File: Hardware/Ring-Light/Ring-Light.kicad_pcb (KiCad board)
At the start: 2 copper layers, 132 x 132 mm, 154 parts, among them Q1 MMBT3904, Q10 MMBT3904, Q11 MMBT3904, Q12 MMBT3904, Q13 MMBT3904, Q14 MMBT3904, Q15 MMBT3904, Q16 MMBT3904, Q2 MMBT3904, Q3 MMBT3904, Q4 MMBT3904, Q5 MMBT3904, Q6 MMBT3904, Q7 MMBT3904, Q8 MMBT3904, Q9 MMBT3904, U1 TPS92612QDBVRQ1, U10 TPS92612QDBVRQ1, U11 TPS92612QDBVRQ1, U12 TPS92612QDBVRQ1, U13 TPS92612QDBVRQ1, U14 TPS92612QDBVRQ1, U15 TPS92612QDBVRQ1, U16 TPS92612QDBVRQ1, U2 TPS92612QDBVRQ1, U3 TPS92612QDBVRQ1, U4 TPS92612QDBVRQ1, U5 TPS92612QDBVRQ1, U6 TPS92612QDBVRQ1, U7 TPS92612QDBVRQ1, U8 TPS92612QDBVRQ1, U9 TPS92612QDBVRQ1

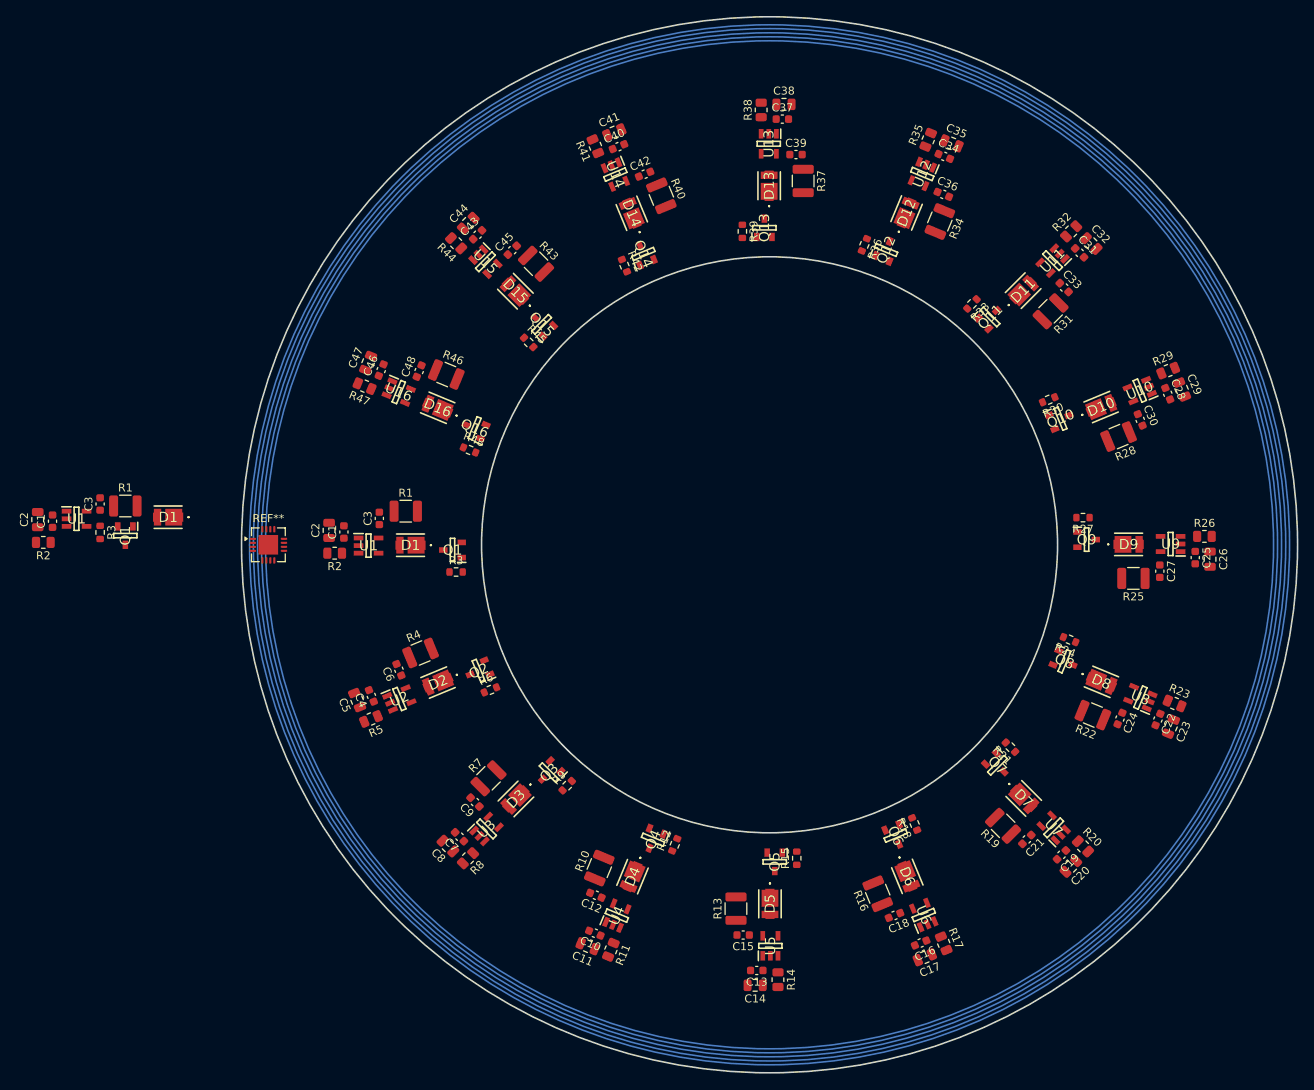
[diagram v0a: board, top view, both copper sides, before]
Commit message: m
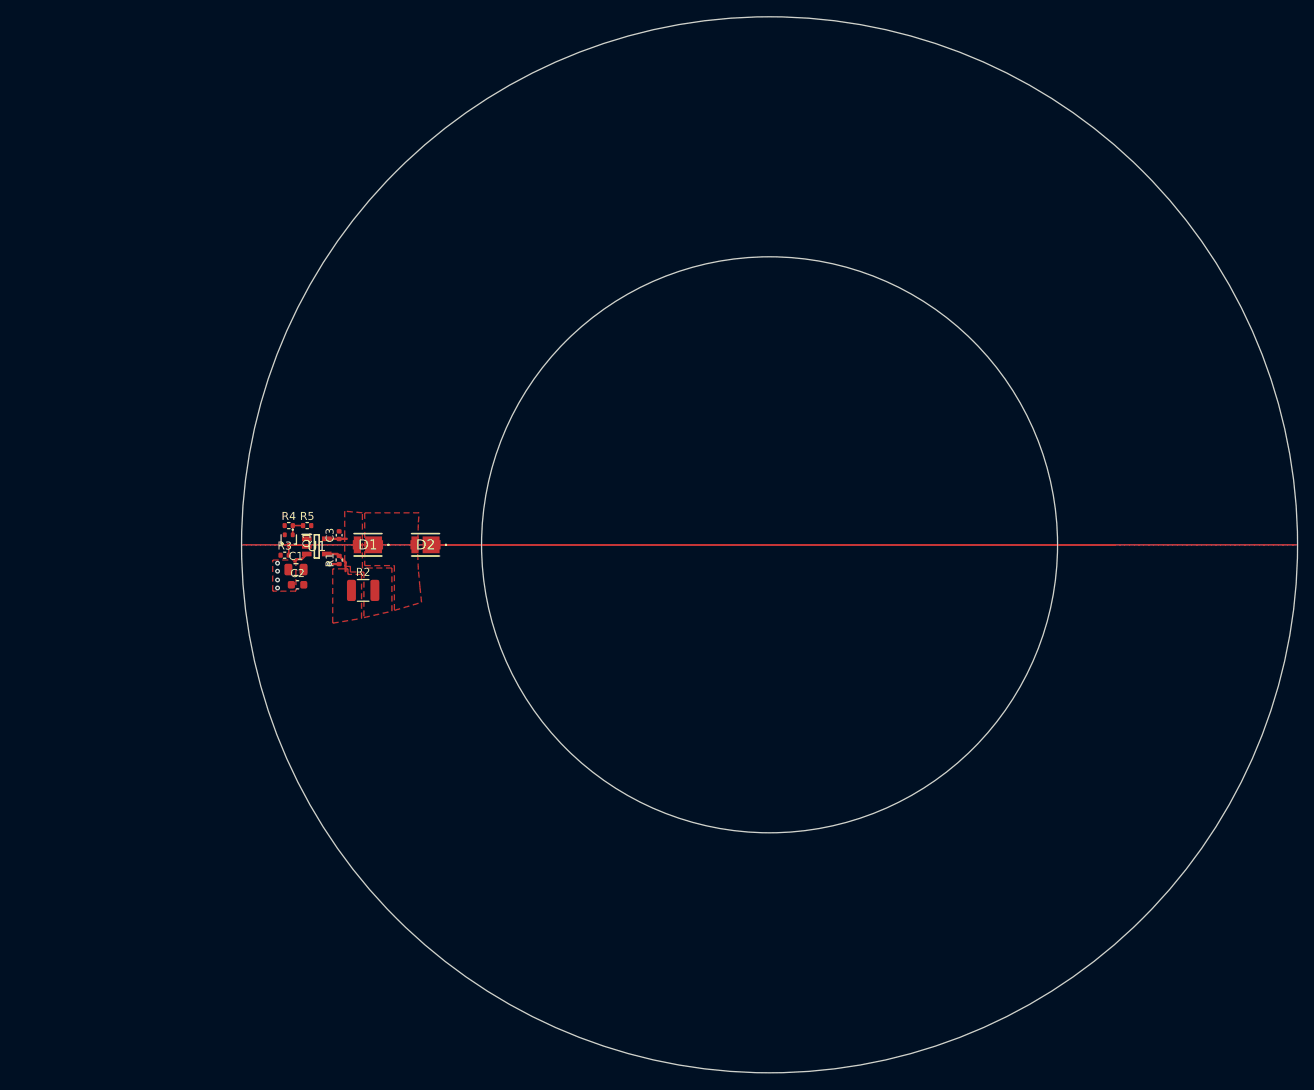
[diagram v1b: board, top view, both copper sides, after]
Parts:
- removed the C1 at (10.4, 97.0)
- removed the C1 at (46.8, 98.4)
- removed C10, C13, C16, C19, C22, C25, C28, C31, C34, C37, C4, C40, C43, C46, C7: 0.1uF, Capacitor_SMD:C_0603_1608Metric
- removed C11, C14, C17, C20, C23, C26, C29, C32, C35, C38, C41, C44, C47, C5, C8: 1uF, Capacitor_SMD:C_0805_2012Metric
- removed C12, C15, C18, C21, C24, C27, C30, C33, C36, C39, C42, C45, C48, C6, C9: 10nF, Capacitor_SMD:C_0603_1608Metric
- removed the C2 at (8.52, 96.8)
- removed the C2 at (44.9, 98.2)
- removed the C3 at (16.3, 94.9)
- removed the C3 at (51.2, 96.7)
- removed the D1 at (55.1, 100.0)
- removed the D1 at (24.8, 96.5)
- removed D10, D11, D12, D13, D14, D15, D16, D3, D4, D5, D6, D7, D8, D9: LED, Library:GWJTLRS1EMLVL5XX531
- removed the Q1 at (19.5, 98.8)
- removed the Q1 at (60.4, 100.7)
- removed Q10, Q11, Q12, Q13, Q14, Q15, Q16, Q2, Q3, Q4, Q5, Q6, Q7, Q8, Q9: MMBT3904, Library:SOT95P240X120-3N
- removed the R1 at (54.5, 95.8)
- removed the R1 at (19.5, 95.2)
- removed R10, R13, R16, R19, R22, R25, R28, R31, R34, R37, R40, R43, R46, R7: 102, Resistor_SMD:R_1210_3225Metric
- removed R11, R14, R17, R20, R23, R26, R29, R32, R35, R38, R41, R44, R47, R8: 0.1, Resistor_SMD:R_0805_2012Metric
- removed R12, R15, R18, R21, R24, R27, R30, R33, R36, R39, R42, R45, R48, R6, R9: 270, Resistor_SMD:R_0603_1608Metric
- removed the R2 at (9.22, 99.7)
- removed the R2 at (45.6, 101.0)
- removed the R3 at (16.3, 98.5)
- removed the R3 at (60.8, 103.4)
- removed REF**: QFN-16-1EP_4x4mm_P0.5mm_EP2.45x2.45mm, Package_DFN_QFN:QFN-16-1EP_4x4mm_P0.5mm_EP2.45x2.45mm
- removed the U1 at (13.4, 96.8)
- removed the U1 at (49.9, 100.1)
- removed U10, U11, U12, U13, U14, U15, U16, U2, U3, U4, U5, U6, U7, U8, U9: TPS92612QDBVRQ1, Library:SOT95P280X145-5N
- added C1: 1uF, Capacitor_SMD:C_0805_2012Metric, F.Cu at (40.8, 103.1)
- added C2: 0.1uF, Capacitor_SMD:C_0603_1608Metric, F.Cu at (41.0, 105.0)
- added C3: 10nF, Capacitor_SMD:C_0402_1005Metric, F.Cu at (46.2, 98.8)
- added D1: LED, Library:GWJTLRS1EMLVL5XX531, F.Cu at (49.8, 100.0)
- added Q1: MMBT3904, Package_TO_SOT_SMD:SOT-416, F.Cu at (39.9, 99.4)
- added R1: 1, Resistor_SMD:R_0402_1005Metric, F.Cu at (46.2, 101.9)
- added R2: 80.6, Resistor_SMD:R_1210_3225Metric, F.Cu at (49.2, 105.7)
- added R3: 1k, Resistor_SMD:R_0402_1005Metric, F.Cu at (39.4, 101.3)
- added U1: TPS92612QDBVRQ1, Library:SOT95P280X145-5N, F.Cu at (43.4, 100.2)
- R4: value 102 -> 10k; footprint Resistor_SMD:R_1210_3225Metric -> Resistor_SMD:R_0402_1005Metric
- R5: value 0.1 -> 10k; footprint Resistor_SMD:R_0805_2012Metric -> Resistor_SMD:R_0402_1005Metric
- moved R5 25.5 mm to (42.2, 97.6), turned to 0 degrees
- moved R4 22.9 mm to (39.9, 97.6), turned to 0 degrees
- moved D2 17.3 mm to (57.0, 100.0), turned to 180 degrees
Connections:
- D2 pad 1: Net-(Q1-C) -> GND
- D2 pad 2: Net-(Q1-C) -> GND
- D2 pad 3: Net-(U1-OUT) -> /LED1
- D2 pad 4: Net-(U1-OUT) -> /LED1
- R4 pad 1: Net-(U1-IN) -> EN1
- R4 pad 2: Net-(U1-OUT) -> /B1
- R5 pad 1: +12V -> /B1
- R5 pad 2: Net-(U1-IN) -> GND
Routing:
- net /IN1: track 0.00 -> 3.89 mm
- net /PWM1: track 0.00 -> 3.56 mm
- net +12V: track 0.00 -> 3.15 mm, vias 0 -> 5
- net /OUT1: track 0.00 -> 2.54 mm
- net /B1: track 0.00 -> 2.43 mm
- added copper zone on F.Cu, net +12V
- added copper zone on F.Cu, net /IN1
- added copper zone on F.Cu, net /LED1
- added copper zone on F.Cu, net /OUT1
- added copper zone on B.Cu, net GND
- added copper zone on F.Cu, net GND
- added copper zone on In1.Cu, net GND
- added copper zone on In2.Cu, net GND
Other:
- copper layers 2 -> 4
